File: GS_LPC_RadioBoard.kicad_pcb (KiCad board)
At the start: 2 copper layers, 30 x 27 mm, 19 parts, among them J1 142-0701-886, J3 Conn_01x04_Pin, J4 Conn_01x07_Pin, Y1 NX2016SA-26M-STD-CZS-1

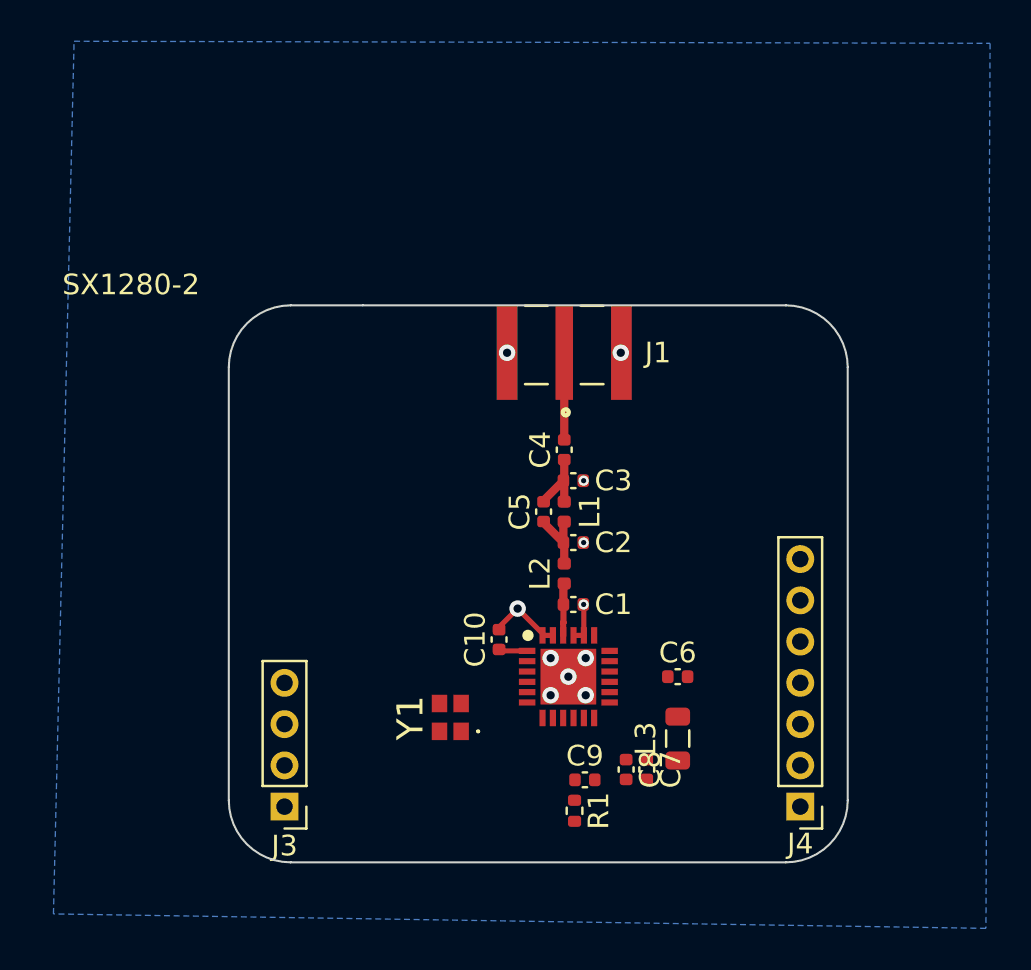
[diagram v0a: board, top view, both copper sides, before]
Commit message: finish first wiring
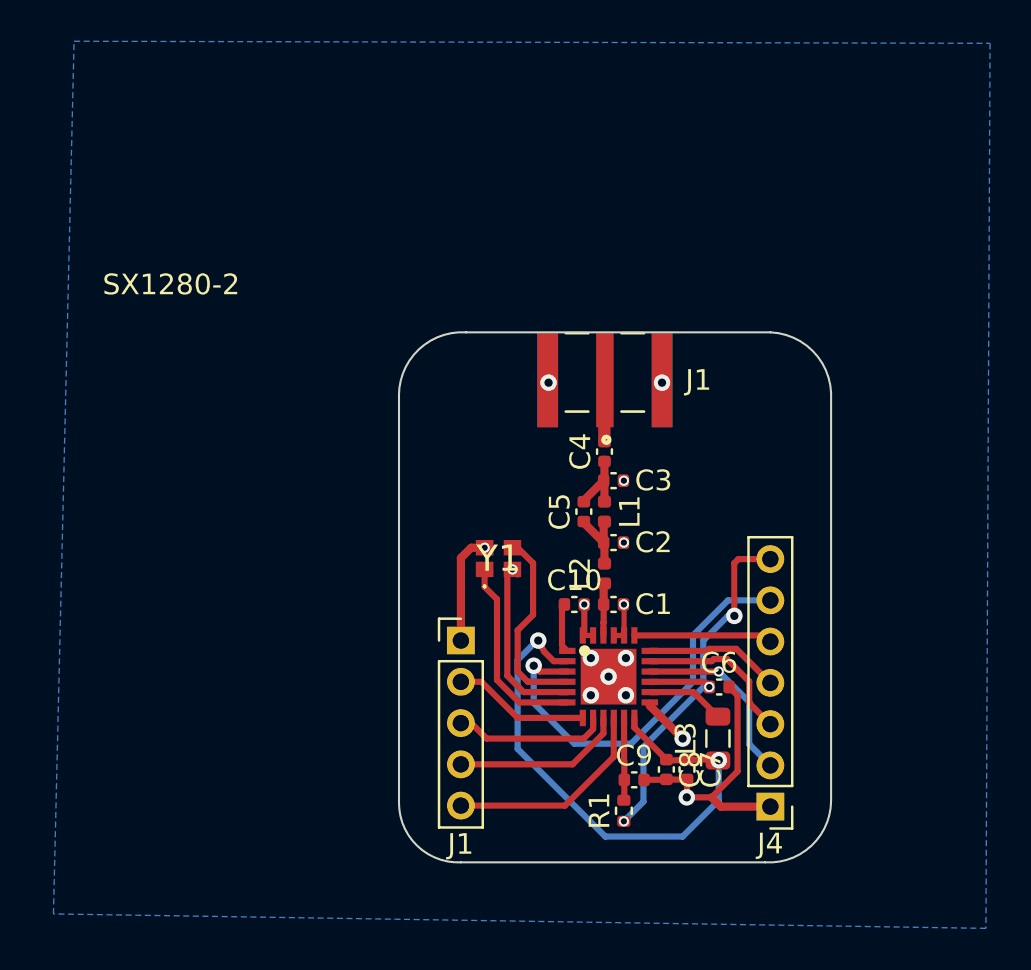
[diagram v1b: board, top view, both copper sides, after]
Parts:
- removed J3: Conn_01x04_Pin, Connector_PinHeader_2.00mm:PinHeader_1x04_P2.00mm_Vertical
- added J1: Conn_01x05_Pin, Connector_PinHeader_2.00mm:PinHeader_1x05_P2.00mm_Vertical, F.Cu at (128.2, 131.8)
- moved Y1 8.05 mm to (130.1, 127.8), turned to 0 degrees
- moved C10 4.03 mm to (133.8, 130.0), turned to 0 degrees
- moved C9 2.39 mm to (136.7, 138.5)
- moved R1 2.39 mm to (136.2, 140.0), turned to 90 degrees
- moved J1 2.38 mm to (135.2, 119.1)
- moved C6 2.07 mm to (140.8, 134.0)
- moved C4 1.95 mm to (135.2, 122.6)
- moved C1 1.95 mm to (135.7, 130.0)
- moved C2 1.95 mm to (135.7, 127.0)
- moved C3 1.95 mm to (135.7, 124.0)
- moved C5 1.95 mm to (134.2, 125.5)
- moved C7 1.95 mm to (139.2, 138.0)
- moved C8 1.95 mm to (138.2, 138.0)
- moved L1 1.95 mm to (135.2, 125.5)
- moved L2 1.95 mm to (135.2, 128.5)
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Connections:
- J1 pad SH1: (no net) -> GND
- J1 pad SH2: (no net) -> GND
- J1 pad SH3: (no net) -> GND
- J1 pad SH4: (no net) -> GND
- J4 pad 7: GND -> /VDD_RADIO
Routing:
- net GND: track 5.70 -> 33.9 mm, vias 9 -> 15
- net /V_DCC: track 0.00 -> 27.2 mm, vias 0 -> 2
- net /NRESET: track 0.00 -> 20.3 mm, vias 0 -> 1
- net /VDD_RADIO: track 0.00 -> 20.1 mm, vias 0 -> 3
- net /DIO3: track 0.00 -> 10.5 mm
- net /XTA: track 0.00 -> 9.49 mm
- net Net-(SX1280-2-XTB): track 0.00 -> 9.47 mm
- net /MISO_TX: track 0.00 -> 8.93 mm, vias 0 -> 1
- net /DIO2: track 0.00 -> 8.49 mm
- net /MOSI_RX: track 0.00 -> 7.80 mm
- net /DIO1: track 0.00 -> 7.45 mm
- net /NSS_CTS: track 0.00 -> 7.00 mm
- net /SCK: track 0.00 -> 6.57 mm
- net /BUSY: track 0.00 -> 6.13 mm
- net Net-(SX1280-2-VBAT_IO): track 0.00 -> 4.02 mm
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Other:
- board size 30 x 27 mm -> 20.9 x 25.7 mm

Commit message: version with minor adjustement
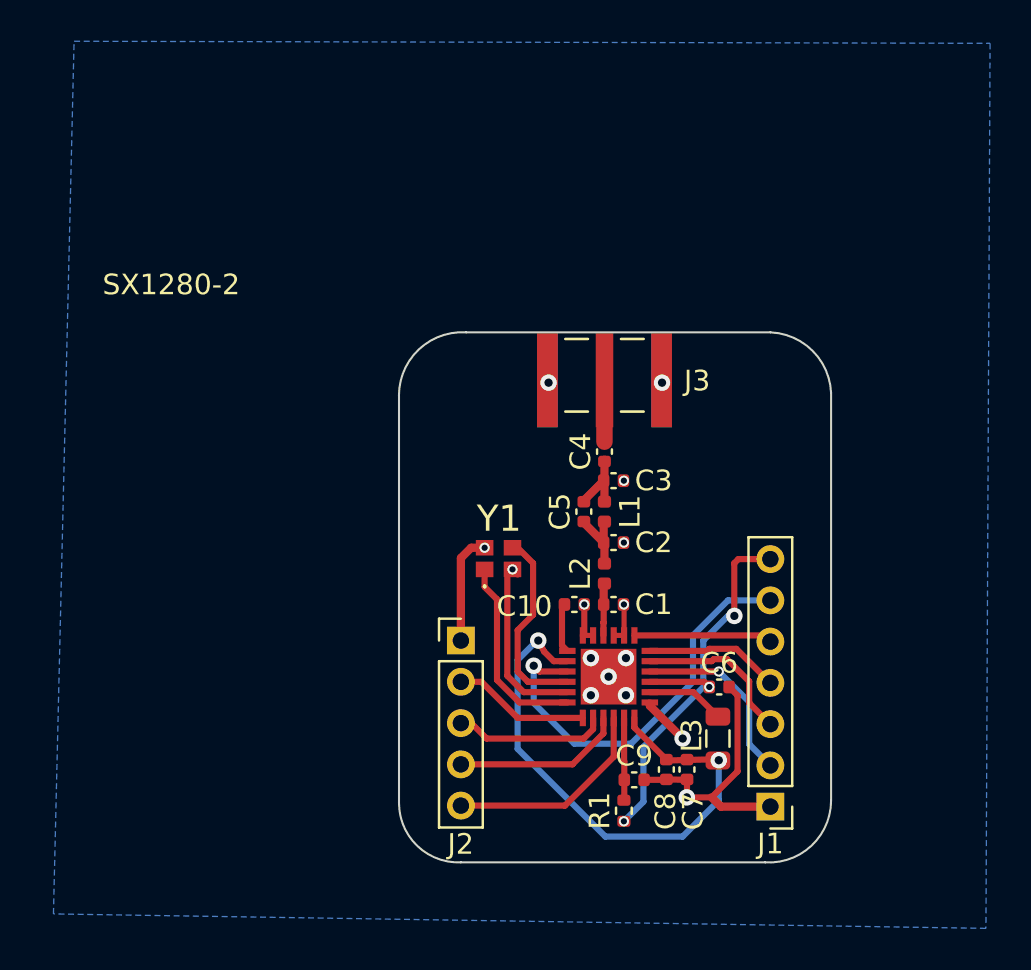
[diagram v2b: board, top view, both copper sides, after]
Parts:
- removed the J1 at (135.2, 119.1)
- added J3: EMPCB.SMAFSTJ.B.HT, footprints:TAOGLAS_EMPCB.SMAFSTJ.B.HT, F.Cu at (135.2, 119.1)
- renumbered J4 to J1, J1 to J2
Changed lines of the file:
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@@
   (net 20 "/XTA")
   (net 21 "Net-(SX1280-2-XTB)")
+  (footprint "footprints:TAOGLAS_EMPCB.SMAFSTJ.B.HT" (layer "F.Cu")
+    (at 135.20925 119.13 180)
+    (property "MANUFACTURER" "TAOGLAS")
+    (property "STANDARD" "Manufacturer Recommendation")
+    (property "Sheetfile" "GS_LPC_RadioBoard.kicad_sch")
+    (property "Sheetname" "")
+    (attr through_hole)
+    (fp_text reference "J3" (at -4.49075 -0.03) (layer "F.SilkS")
+        (effects (font (size 1.000961 1.000961) (thickness 0.15)))
+    )
+    (fp_text value "EMPCB.SMAFSTJ.B.HT" (at 13.20051 12.745575) (layer "F.Fab")
+        (effects (font (size 1.000039 1.000039) (thickness 0.15)))
+    )
+    (fp_text user "PCB EDGE" (at 3.80679 2.10375) (layer "F.Fab")
+        (effects (font (size 0.320572 0.320572) (thickness 0.15)))
+    )
+    (fp_line (start -1.9 -1.52) (end -0.8 -1.52)
+      (stroke (width 0.127) (type solid)) (layer "F.SilkS"))
+    (fp_line (start -1.9 2) (end -0.8 2)
+      (stroke (width 0.127) (type solid)) (layer "F.SilkS"))
+    (fp_line (start 0.8 -1.52) (end 1.9 -1.52)
+      (stroke (width 0.127) (type solid)) (layer "F.SilkS"))
+    (fp_line (start 0.8 2) (end 1.9 2)
+      (stroke (width 0.127) (type solid)) (layer "F.SilkS"))
+    (fp_line (start -3.52 -2.53) (end 3.52 -2.53)
+      (stroke (width 0.05) (type solid)) (layer "B.CrtYd"))
+    (fp_line (start -3.52 12.03) (end -3.52 -2.53)
+      (stroke (width 0.05) (type solid)) (layer "B.CrtYd"))
+    (fp_line (start 3.52 -2.53) (end 3.52 12.03)
+      (stroke (width 0.05) (type solid)) (layer "B.CrtYd"))
+    (fp_line (start 3.52 12.03) (end -3.52 12.03)
+      (stroke (width 0.05) (type solid)) (layer "B.CrtYd"))
+    (fp_line (start -3.52 -2.53) (end 3.52 -2.53)
+      (stroke (width 0.05) (type solid)) (layer "F.CrtYd"))
+    (fp_line (start -3.52 12.03) (end -3.52 -2.53)
+      (stroke (width 0.05) (type solid)) (layer "F.CrtYd"))
+    (fp_line (start 3.52 -2.53) (end 3.52 12.03)
+      (stroke (width 0.05) (type solid)) (layer "F.CrtYd"))
+    (fp_line (start 3.52 12.03) (end -3.52 12.03)
+      (stroke (width 0.05) (type solid)) (layer "F.CrtYd"))
+    (fp_line (start -3.175 -1.52) (end 3.175 -1.52)
+      (stroke (width 0.127) (type solid)) (layer "F.Fab"))
+    (fp_line (start -3.175 2.28) (end -3.175 -1.52)
+      (stroke (width 0.127) (type solid)) (layer "F.Fab"))
+    (fp_line (start -3.175 2.28) (end 5 2.28)
+      (stroke (width 0.127) (type solid)) (layer "F.Fab"))
+    (fp_line (start -3.175 11.78) (end -3.175 2.28)
+      (stroke (width 0.127) (type solid)) (layer "F.Fab"))
+    (fp_line (start 3.175 -1.52) (end 3.175 11.78)
+      (stroke (width 0.127) (type solid)) (layer "F.Fab"))
+    (fp_line (start 3.175 11.78) (end -3.175 11.78)
+      (stroke (width 0.127) (type solid)) (layer "F.Fab"))
+    (pad "1" smd rect (at 0 0 180) (size 0.85 4.56) (layers "F.Cu" "F.Paste" "F.Mask")
+      (net 5 "Net-(C4-Pad2)") (pintype "passive"))
+    (pad "SH1" smd rect (at -2.77 0 180) (size 1 4.56) (layers "F.Cu" "F.Paste" "F.Mask")
+      (net 1 "GND") (pintype "passive"))
+    (pad "SH2" smd rect (at 2.77 0 180) (size 1 4.56) (layers "F.Cu" "F.Paste" "F.Mask")
+      (net 1 "GND"))
+    (pad "SH3" smd rect (at -2.77 0 180) (size 1 4.56) (layers "B.Cu" "B.Paste" "B.Mask")
+      (net 1 "GND"))
+    (pad "SH4" smd rect (at 2.77 0 180) (size 1 4.56) (layers "B.Cu" "B.Paste" "B.Mask")
+      (net 1 "GND"))
+  )
   (footprint "Inductor_SMD:L_0402_1005Metric" (layer "F.Cu")
     (at 135.20925 125.5 90)
@@
     (property "ki_keywords" "cap capacitor")
     (attr smd)
-    (fp_text reference "C8" (at 0 -1.16 90) (layer "F.SilkS")
+    (fp_text reference "C8" (at 2.02 0.03925 90) (layer "F.SilkS")
         (effects (font (size 1 1) (thickness 0.15)))
     )
@@
     (property "ki_keywords" "connector")
     (attr through_hole)
-    (fp_text reference "J1" (at -0.01 9.87) (layer "F.SilkS")
+    (fp_text reference "J2" (at -0.01 9.87) (layer "F.SilkS")
         (effects (font (size 1 1) (thickness 0.15)))
     )
@@
     (property "ki_keywords" "cap capacitor")
     (attr smd)
-    (fp_text reference "C10" (at 0 -1.16) (layer "F.SilkS")
+    (fp_text reference "C10" (at -2.42 0.09) (layer "F.SilkS")
         (effects (font (size 1 1) (thickness 0.15)))
     )
@@
     (property "ki_keywords" "cap capacitor")
     (attr smd)
-    (fp_text reference "C7" (at 0 -1.16 90) (layer "F.SilkS")
+    (fp_text reference "C7" (at 2.03 -0.29075 90) (layer "F.SilkS")
         (effects (font (size 1 1) (thickness 0.15)))
     )
@@
     (property "ki_description" "NDK 26MHz Crystal Unit +/-15ppm SMD 4-Pin 2 x 1.6 x 0.45mm")
     (attr smd)
-    (fp_text reference "Y1" (at 0 0) (layer "F.SilkS")
+    (fp_text reference "Y1" (at 0.025 -1.935) (layer "F.SilkS")
         (effects (font (size 1.27 1.27) (thickness 0.254)))
     )
@@
     (property "ki_keywords" "inductor choke coil reactor magnetic")
     (attr smd)
-    (fp_text reference "L3" (at 0 -1.55 90) (layer "F.SilkS")
+    (fp_text reference "L3" (at 0.15 -1.26925 90) (layer "F.SilkS")
         (effects (font (size 1 1) (thickness 0.15)))
     )
@@
     )
   )
-  (footprint "footprints:TAOGLAS_EMPCB.SMAFSTJ.B.HT" (layer "F.Cu")
-    (at 135.23 119.13 180)
-    (property "MANUFACTURER" "Cinch Connectivity")
-    (property "MAXIMUM_PACKAGE_HEIGHT" "8.052 mm")
-    (property "PARTREV" "4a")
-    (property "STANDARD" "Manufacturer Recommendations")
-    (property "Sheetfile" "GS_LPC_RadioBoard.kicad_sch")
-    (property "Sheetname" "")
-    (attr through_hole)
-    (fp_text reference "J1" (at -4.54075 0) (layer "F.SilkS")
-        (effects (font (size 1.000961 1.000961) (thickness 0.15)))
-    )
-    (fp_text value "142-0701-886" (at 13.20051 12.745575) (layer "F.Fab")
-        (effects (font (size 1.000039 1.000039) (thickness 0.15)))
-    )
-    (fp_text user "PCB EDGE" (at 3.80679 2.10375) (layer "F.Fab")
-        (effects (font (size 0.320572 0.320572) (thickness 0.15)))
-    )
-    (fp_line (start -1.9 -1.52) (end -0.8 -1.52)
-      (stroke (width 0.127) (type solid)) (layer "F.SilkS"))
-    (fp_line (start -1.9 2.28) (end -0.8 2.28)
-      (stroke (width 0.127) (type solid)) (layer "F.SilkS"))
-    (fp_line (start 0.8 -1.52) (end 1.9 -1.52)
-      (stroke (width 0.127) (type solid)) (layer "F.SilkS"))
-    (fp_line (start 0.8 2.28) (end 1.9 2.28)
-      (stroke (width 0.127) (type solid)) (layer "F.SilkS"))
-    (fp_circle (center -0.073 -2.888) (end 0.027 -2.888)
-      (stroke (width 0.3) (type solid)) (fill none) (layer "F.SilkS"))
-    (fp_line (start -3.52 -2.53) (end 3.52 -2.53)
-      (stroke (width 0.05) (type solid)) (layer "B.CrtYd"))
-    (fp_line (start -3.52 12.03) (end -3.52 -2.53)
-      (stroke (width 0.05) (type solid)) (layer "B.CrtYd"))
-    (fp_line (start 3.52 -2.53) (end 3.52 12.03)
-      (stroke (width 0.05) (type solid)) (layer "B.CrtYd"))
-    (fp_line (start 3.52 12.03) (end -3.52 12.03)
-      (stroke (width 0.05) (type solid)) (layer "B.CrtYd"))
-    (fp_line (start -3.52 -2.53) (end 3.52 -2.53)
-      (stroke (width 0.05) (type solid)) (layer "F.CrtYd"))
-    (fp_line (start -3.52 12.03) (end -3.52 -2.53)
-      (stroke (width 0.05) (type solid)) (layer "F.CrtYd"))
-    (fp_line (start 3.52 -2.53) (end 3.52 12.03)
-      (stroke (width 0.05) (type solid)) (layer "F.CrtYd"))
-    (fp_line (start 3.52 12.03) (end -3.52 12.03)
-      (stroke (width 0.05) (type solid)) (layer "F.CrtYd"))
-    (fp_line (start -3.175 -1.52) (end 3.175 -1.52)
-      (stroke (width 0.127) (type solid)) (layer "F.Fab"))
-    (fp_line (start -3.175 2.28) (end -3.175 -1.52)
-      (stroke (width 0.127) (type solid)) (layer "F.Fab"))
-    (fp_line (start -3.175 2.28) (end 5 2.28)
-      (stroke (width 0.127) (type solid)) (layer "F.Fab"))
-    (fp_line (start -3.175 11.78) (end -3.175 2.28)
-      (stroke (width 0.127) (type solid)) (layer "F.Fab"))
-    (fp_line (start 3.175 -1.52) (end 3.175 11.78)
-      (stroke (width 0.127) (type solid)) (layer "F.Fab"))
-    (fp_line (start 3.175 11.78) (end -3.175 11.78)
-      (stroke (width 0.127) (type solid)) (layer "F.Fab"))
-    (pad "1" smd rect (at 0 0 180) (size 0.85 4.56) (layers "F.Cu" "F.Paste" "F.Mask")
-      (net 5 "Net-(C4-Pad2)") (pintype "passive"))
-    (pad "SH1" smd rect (at -2.77 0 180) (size 1 4.56) (layers "F.Cu" "F.Paste" "F.Mask")
-      (net 1 "GND"))
-    (pad "SH2" smd rect (at 2.77 0 180) (size 1 4.56) (layers "F.Cu" "F.Paste" "F.Mask")
-      (net 1 "GND"))
-    (pad "SH3" smd rect (at -2.77 0 180) (size 1 4.56) (layers "B.Cu" "B.Paste" "B.Mask")
-      (net 1 "GND"))
-    (pad "SH4" smd rect (at 2.77 0 180) (size 1 4.56) (layers "B.Cu" "B.Paste" "B.Mask")
-      (net 1 "GND"))
-  )
   (footprint "Connector_PinHeader_2.00mm:PinHeader_1x07_P2.00mm_Vertical" (layer "F.Cu")
     (at 143.25 139.8 180)
@@
     (property "ki_keywords" "connector")
     (attr through_hole)
-    (fp_text reference "J4" (at 0 -1.8) (layer "F.SilkS")
+    (fp_text reference "J1" (at 0 -1.8) (layer "F.SilkS")
         (effects (font (size 1 1) (thickness 0.15)))
     )
@@
     )
   )
-  (gr_circle (center 134.25 132.25) (end 134.45 132.25)
-    (stroke (width 0.15) (type solid)) (fill solid) (layer "F.SilkS"))
   (gr_line (start 146.194361 139.500001) (end 146.194361 119.75)
     (stroke (width 0.1) (type default)) (layer "Edge.Cuts"))
@@
   (segment (start 134.20925 124.96075) (end 135.17 124) (width 0.4) (layer "F.Cu") (net 4))
   (segment (start 135.20925 125.015) (end 135.20925 124.03925) (width 0.4) (layer "F.Cu") (net 4))
-  (segment (start 135.205 119) (end 135.205 121.99925) (width 0.6) (layer "F.Cu") (net 5))
+  (segment (start 135.20925 119.13) (end 135.20925 122.10925) (width 0.8) (layer "F.Cu") (net 5))
+  (segment (start 135.20925 122.10925) (end 135.21 122.11) (width 0.4) (layer "F.Cu") (net 5))
   (segment (start 135.23 121.99925) (end 135.20925 122.02) (width 0.4) (layer "F.Cu") (net 5))
   (segment (start 141.5 128) (end 141.7 127.8) (width 0.3) (layer "F.Cu") (net 6))
